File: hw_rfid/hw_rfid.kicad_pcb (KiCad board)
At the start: 2 copper layers, 46 parts, among them IC1 XC9288A33CER-G, IC2 TPS610333DRLR, J1 Conn_01x02, J2 Conn_01x05, J3 Conn_01x04, J4 Conn_01x03, J5 Conn_01x08, Q1 2N7002, SW1 SW_Push, SW2 SW_Push, SW3 SW_Push, U1 STM32U031K6Ux, U2 AT45DB021E-SHN-T

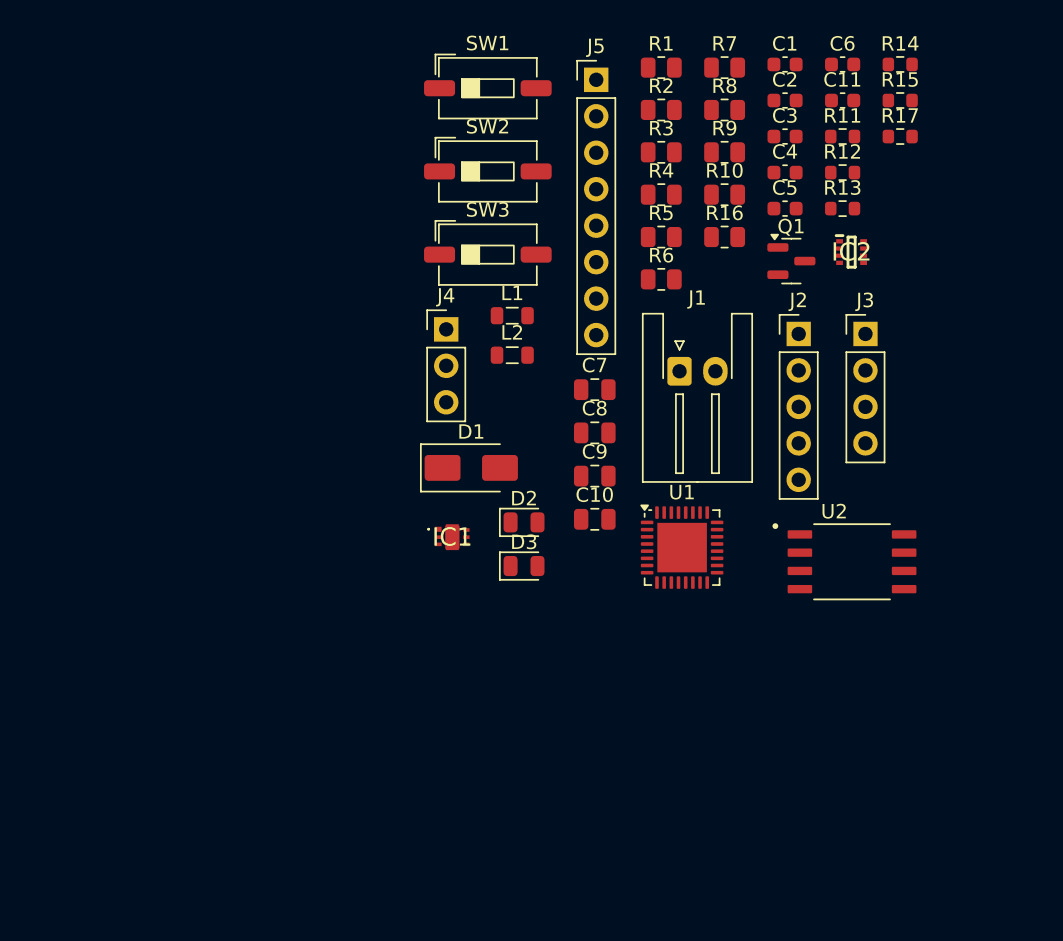
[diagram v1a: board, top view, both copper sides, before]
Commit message: PLACA atualizada
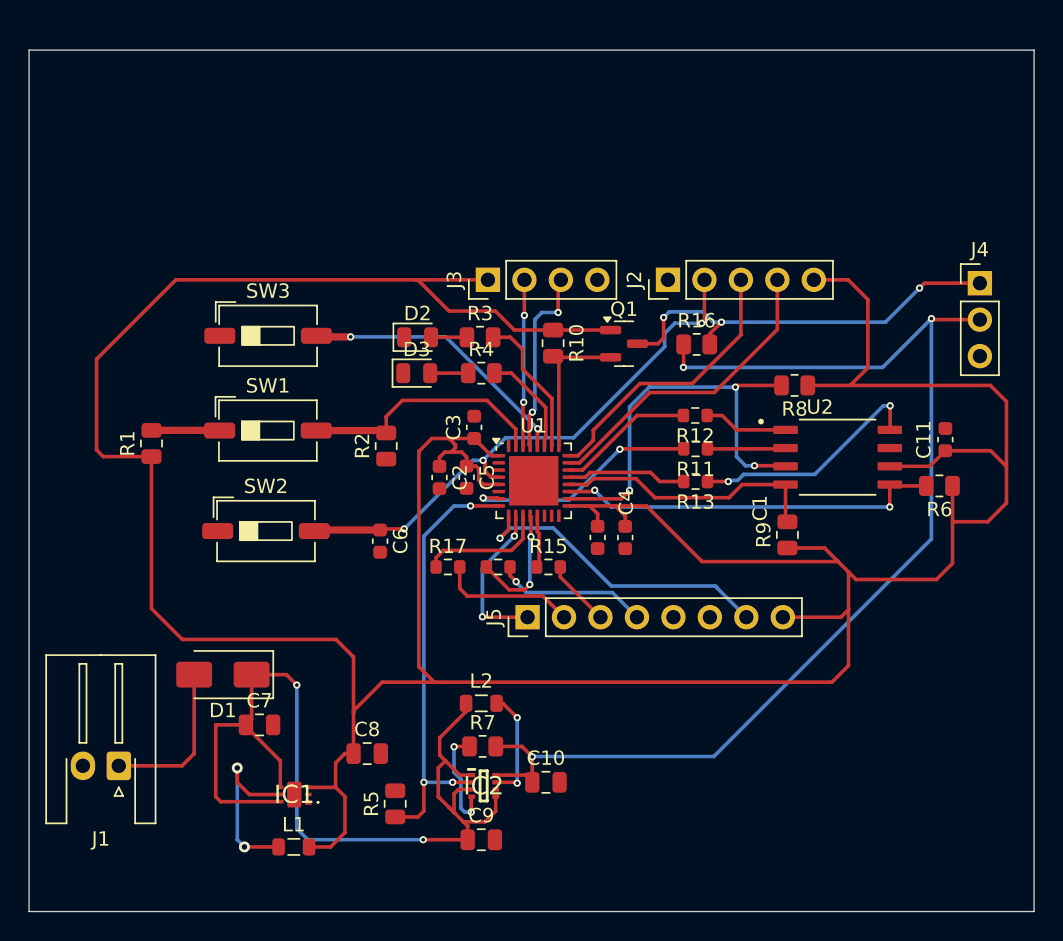
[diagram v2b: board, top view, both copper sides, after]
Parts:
- IC1: footprint XC9288A:USP-6C -> XC9288A33CER-G:USP-6C
- IC2: footprint TPS6103:SOTFL50P160X60-8N -> TPS610333DRLR:SOTFL50P160X60-8N
- U2: footprint AT45DB:SOIC127P798X216-8N -> AT45DB021E-SHN-T:SOIC127P798X216-8N
- moved R7 50.2 mm to (107.1, 114.0)
- moved J1 47.8 mm to (81.8, 115.3), turned to 180 degrees
- moved C6 46.3 mm to (100.0, 99.7), turned to -90 degrees
- moved IC2 45.2 mm to (107.2, 116.8)
- moved R14 44.8 mm to (108.2, 101.5)
- moved R1 44.1 mm to (84.0, 92.9), turned to 90 degrees
- moved R5 43.6 mm to (101.0, 118.0), turned to 90 degrees
- moved R17 43.5 mm to (104.7, 101.5)
- moved R15 40.7 mm to (111.7, 101.5)
- moved L1 40.0 mm to (93.9, 121.0)
- moved J5 37.7 mm to (110.2, 105.0), turned to 90 degrees
- moved J4 37.3 mm to (141.7, 81.7)
- moved C2 35.6 mm to (104.1, 95.3), turned to -90 degrees
- moved C1 34.8 mm to (117.0, 99.5), turned to -90 degrees
- moved C7 33.0 mm to (91.5, 112.5)
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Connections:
- J2 pad 3: /SWDIO -> /SWCLK
- J2 pad 4: /SWCLK -> /SWDIO
- J3 pad 2: /LPUART2_TX -> /LPUART2_RX
- J3 pad 3: /LPUART2_RX -> /LPUART2_TX
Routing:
- net +3.3V: track 0.00 -> 265.3 mm
- net +5V: track 0.00 -> 80.5 mm, vias 0 -> 3
- net +BATT: track 0.00 -> 66.4 mm, vias 0 -> 2
- net /NRST: track 0.00 -> 38.6 mm, vias 0 -> 3
- net /ENABLE_5V_REG: track 0.00 -> 30.7 mm, vias 0 -> 3
- net /nRESET_FLASH: track 0.00 -> 30.1 mm, vias 0 -> 3
- net /AMP_PWM: track 0.00 -> 28.9 mm, vias 0 -> 3
- net /nWP_FLASH: track 0.00 -> 27.1 mm, vias 0 -> 2
- net /nRSTPD_RFID: track 0.00 -> 21.9 mm, vias 0 -> 1
- net /SWDIO: track 0.00 -> 21.8 mm
- net /SWCLK: track 0.00 -> 19.7 mm
- net /PUSH_BUTTON_01: track 0.00 -> 19.3 mm, vias 0 -> 2
- net /nCS_FLASH: track 0.00 -> 18.9 mm
- net /BOOT0: track 0.00 -> 17.6 mm
- net /SPI2_SCK_FLASH: track 0.00 -> 16.7 mm, vias 0 -> 2
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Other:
- board outline added: 70 x 60 mm
